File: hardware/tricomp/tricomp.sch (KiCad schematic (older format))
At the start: 10 parts, among them J1 ISP, J2 Power/i2c, J3 Conn_01x05, J4 Conn_01x05, U1 ATMEGA328P-PU, Y1 Crystal

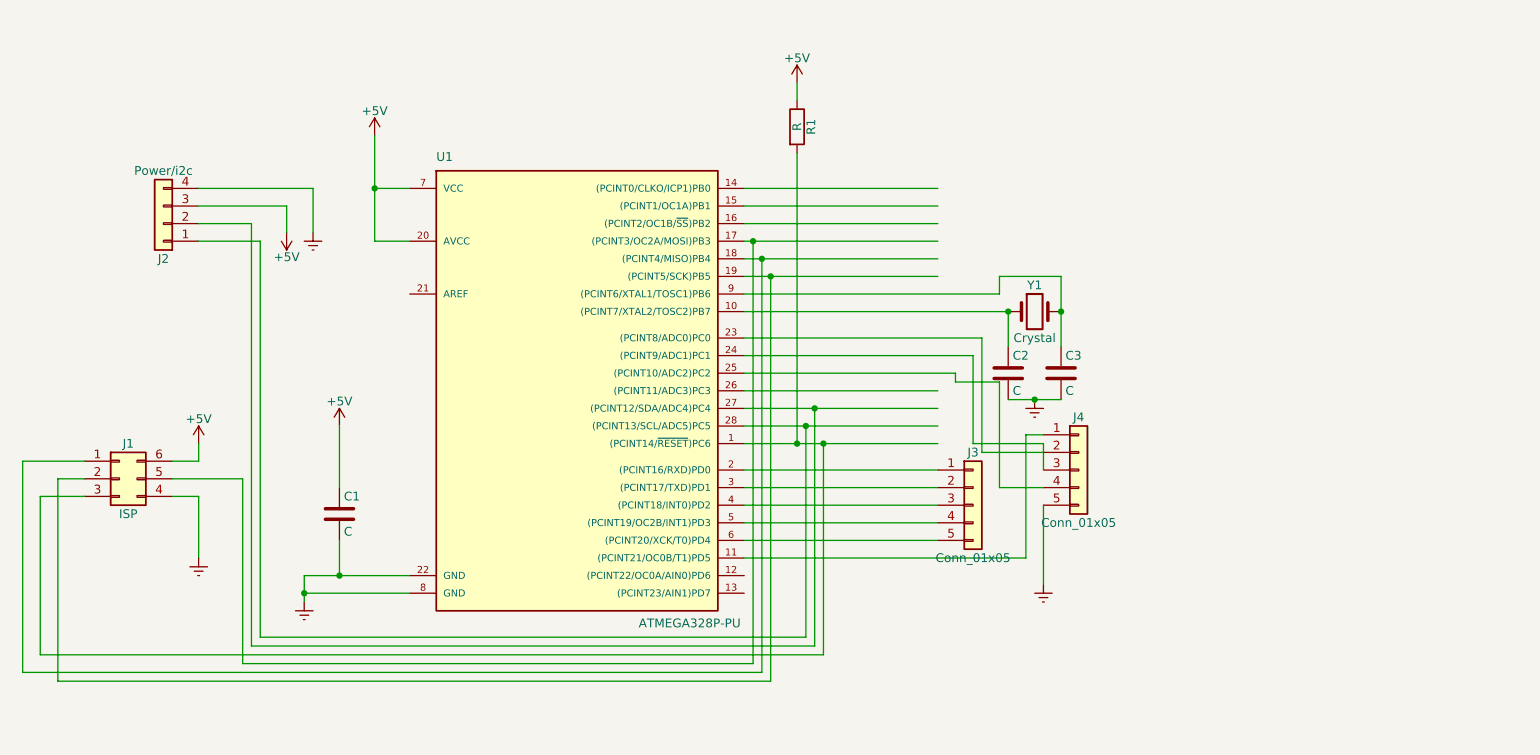
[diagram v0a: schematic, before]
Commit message: building stripboard prototype
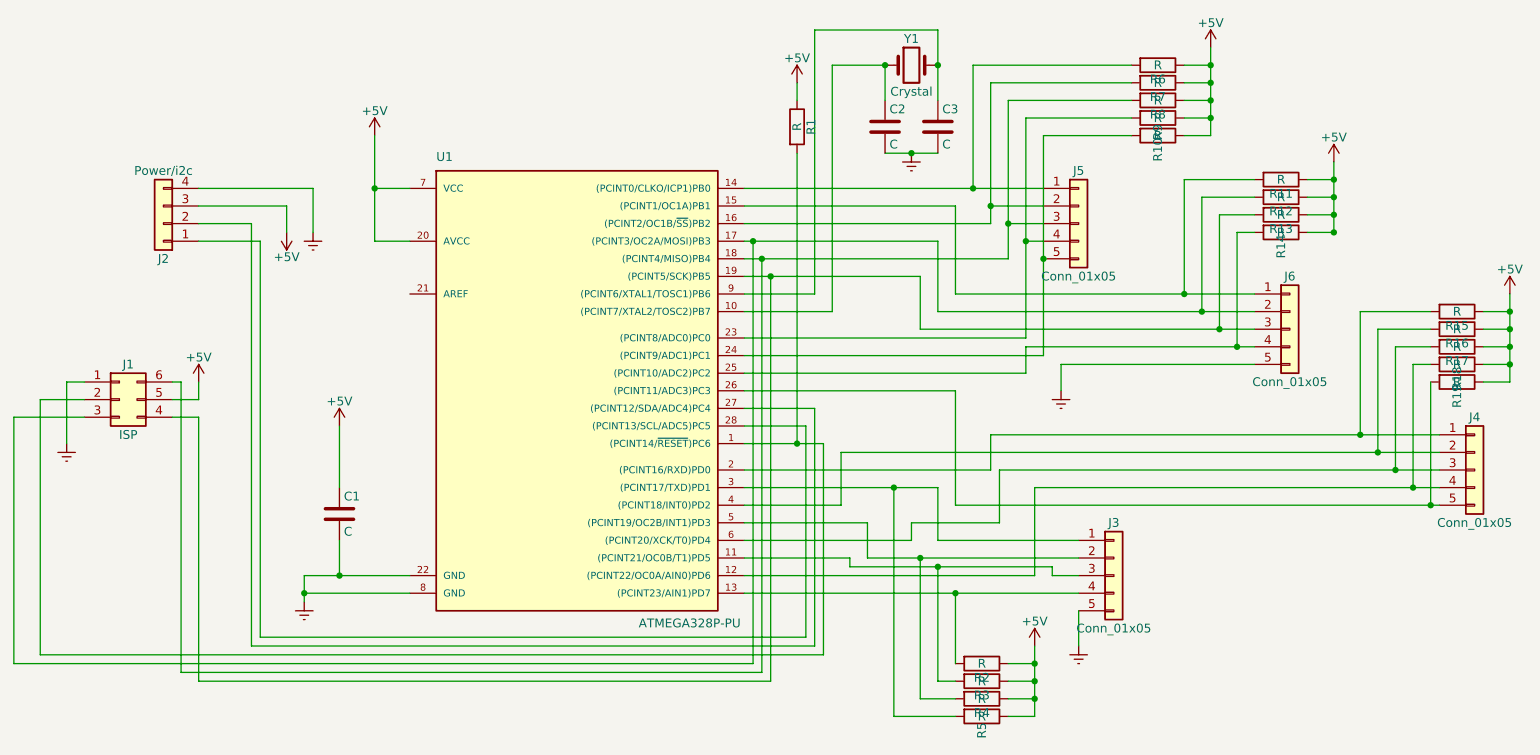
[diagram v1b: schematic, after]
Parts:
- added J5, J6: Conn_01x05, Pin_Headers:Pin_Header_Straight_1x05_Pitch2.54mm, symbol Conn_01x05
- added R10, R11, R12, R13, R14, R15, R16, R17, R18, R19, R2, R3, R4, R5, R6, R7, R8, R9: R, Resistors_THT:R_Axial_DIN0204_L3.6mm_D1.6mm_P7.62mm_Horizontal, symbol R
- Y1: footprint Crystals:Crystal_HC52-8mm_Vertical -> Connectors_Terminal_Blocks:TerminalBlock_bornier-2_P5.08mm
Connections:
- wire segments 80 -> 162
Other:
- moved on the sheet: C2, C3, J1, J3, J4, Y1
